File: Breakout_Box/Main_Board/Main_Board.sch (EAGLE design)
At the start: 31 parts, among them CN1 19PIN_LEMO, Q1 DMP3099L, Q2 DSS6060

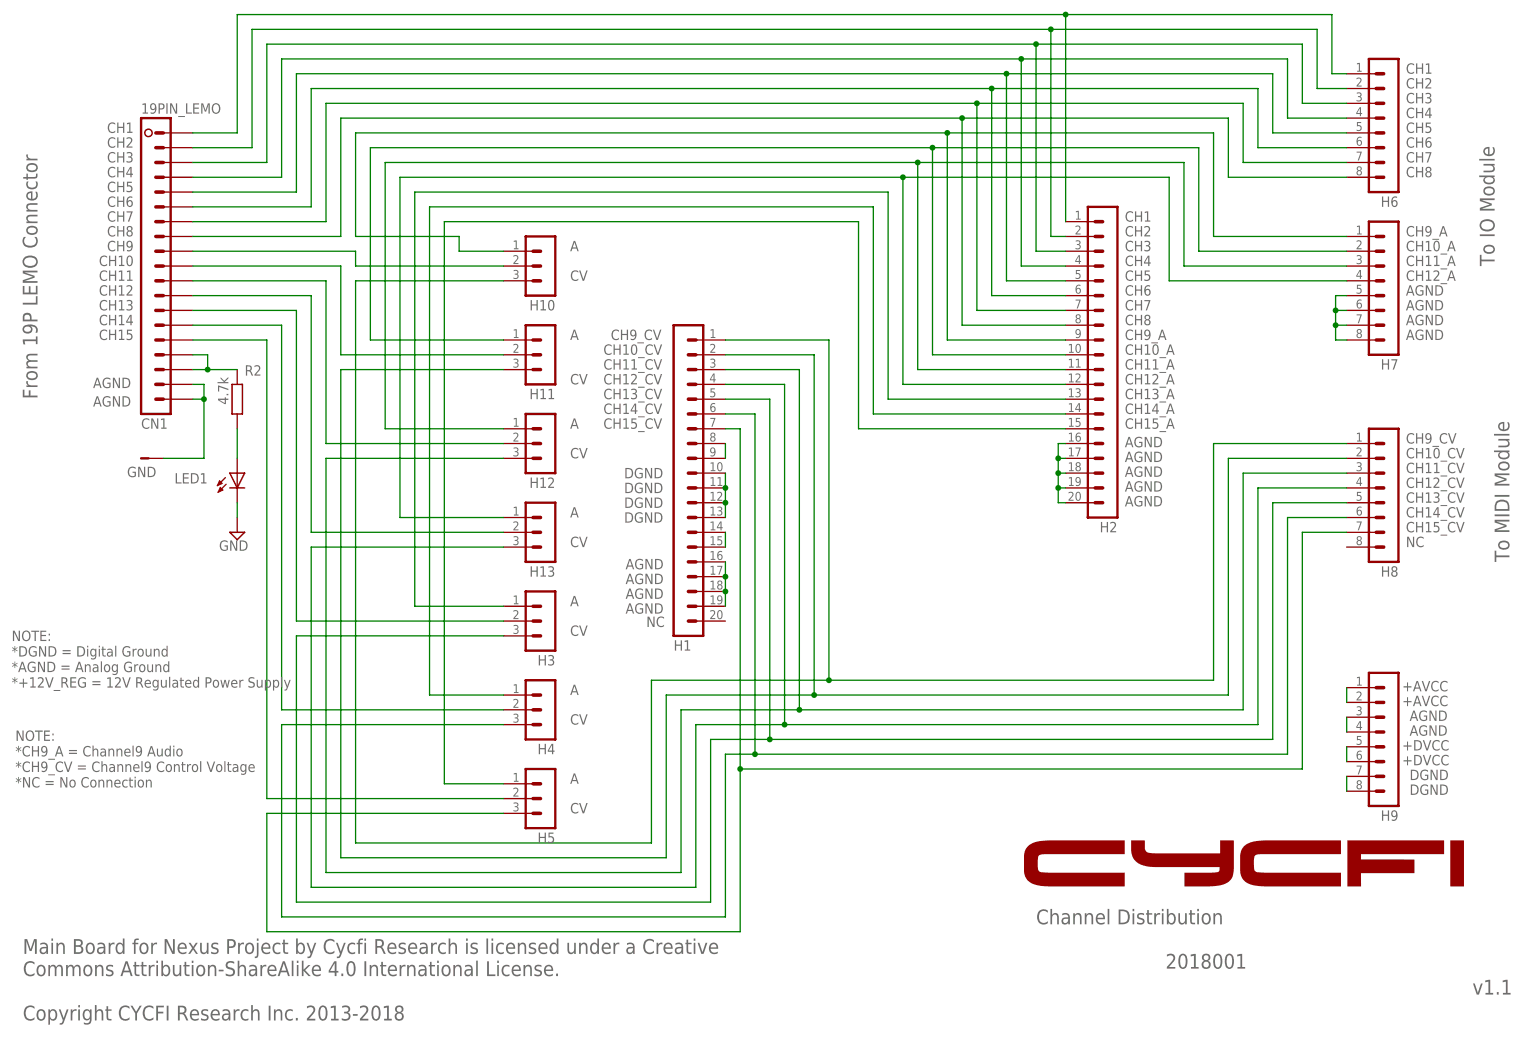
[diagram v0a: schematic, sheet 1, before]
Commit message: merge version_1.1 to devel
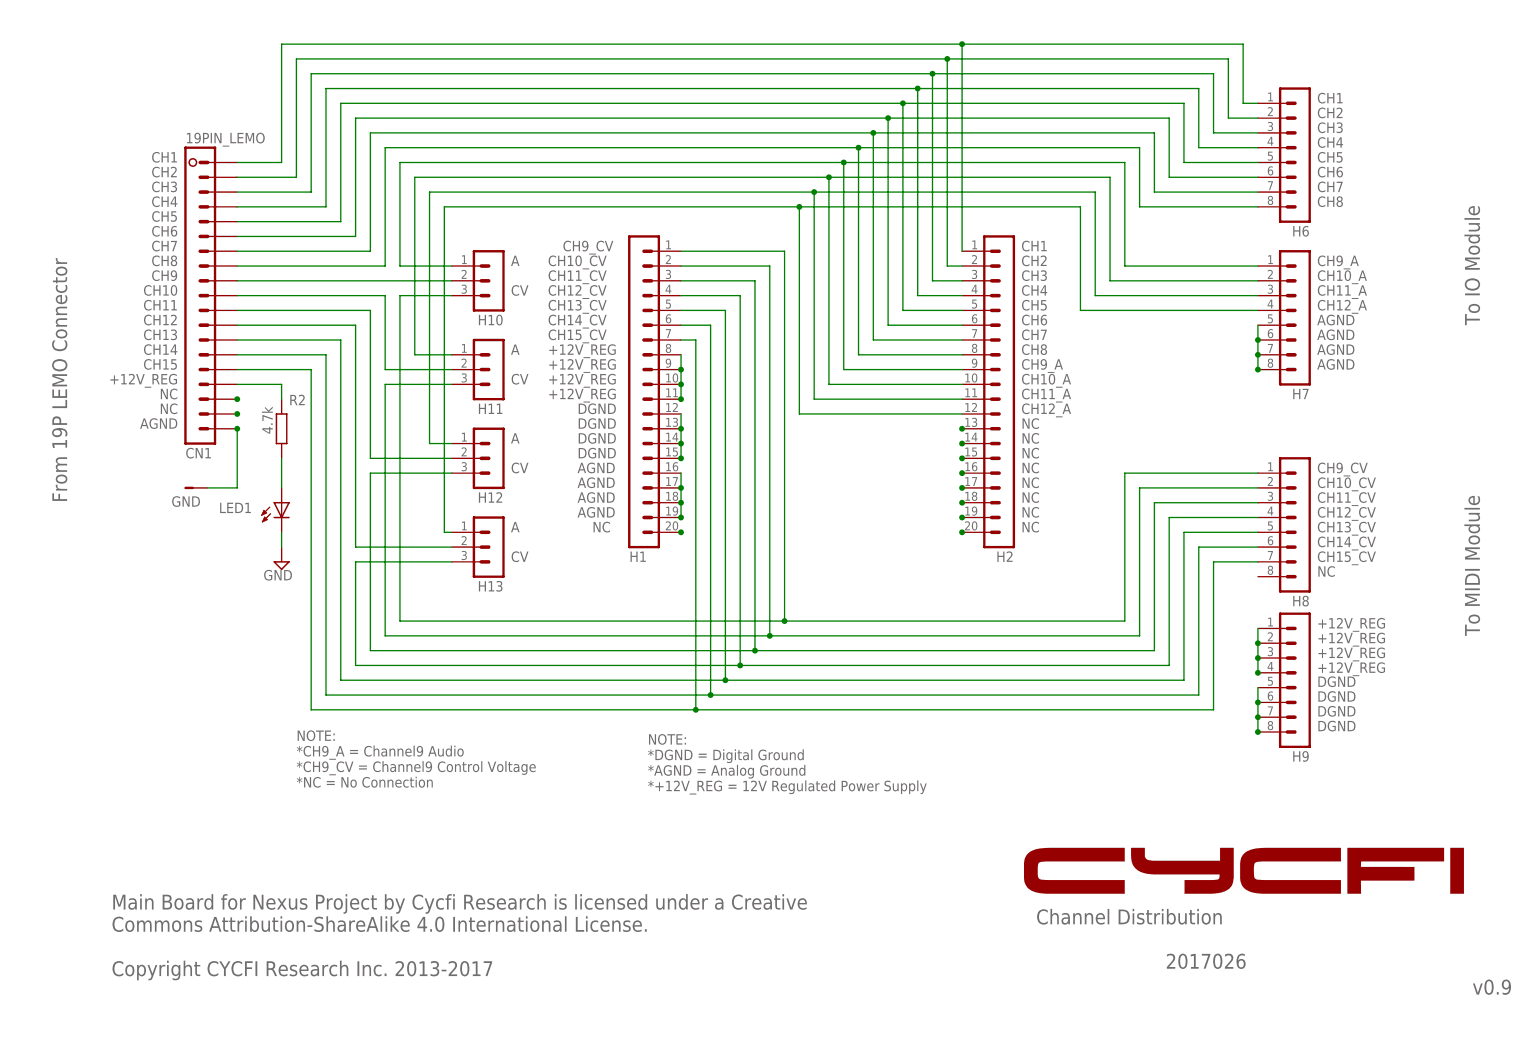
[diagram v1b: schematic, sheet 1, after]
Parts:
- removed C1, C3: 22uF, resistor:C-EUC0805
- removed C4: 1uF, resistor:C-EUC0603
- removed C5: 10uF, resistor:C-EUC0603
- removed C7: 1nF, resistor:C-EUC0402K
- removed H3, H4, H5: (no value), con-lstb:MA03-1_EDITED
- removed L2: 82uH, resistor:L-EU
- removed Q1: DMP3099L, CYCFI_semicon:P_MOSFET
- removed Q2: DSS6060, CYCFI_semicon:DSS60601MZ4-13
- removed R1: 1k, resistor:R-EU_R0402
- C2: value 470uF -> 0.1uF; device resistor:CPOL-EU140CLH-1010 -> resistor:C-EUC0603
- D1: value FM4004W -> FM4007W
- L1: value 1mH -> 100uH; device inductors:SDR -> resistor:L-EU
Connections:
- removed net +AVCC: C4.1, C5.1, C7.1, CN1.16, CN1.17, D1.A, H1.14, H1.15, H9.1, H9.2, Q2.E, R2.1
- removed net +DVCC: C3.1, H1.8, H1.9, H9.5, H9.6, L1.2
- removed net GND: C1.2, C2.-, C3.2, C4.2, C5.2, C6.-, C7.2, CN1.18, CN1.19, GND.P, H1.10, H1.11, H1.12, H1.13, H1.16, H1.17, H1.18, H1.19, H14.1, H2.16, H2.17, H2.18, H2.19, H2.20, H7.5, H7.6, H7.7, H7.8, H9.3, H9.4, H9.7, H9.8, LED1.C, Q1.G
- removed net N$33: H1.5, H3.3, H8.5
- removed net N$34: H1.6, H4.3, H8.6
- removed net N$35: H1.7, H5.3, H8.7
- removed net N$36: CN1.13, H3.2
- removed net N$37: CN1.14, H4.2
- removed net N$38: CN1.15, H5.2
- new net +12V_REG: C2.1, C6.+, CN1.16, H1.10, H1.11, H1.8, H1.9, H9.1, H9.2, H9.3, H9.4, L1.2, R2.1
- new net AGND: C2.2, C6.-, CN1.19, GND.P, H1.16, H1.17, H1.18, H1.19, H14.1, H7.5, H7.6, H7.7, H7.8, LED1.C
- new net DGND: H1.12, H1.13, H1.14, H1.15, H9.5, H9.6, H9.7, H9.8
- new net N$22: H2.19
- new net N$23: H2.20
- new net N$24: H1.20
- new net N$26: CN1.18
- new net N$31: D1.C, L1.1
- new net N$60: CN1.13, H1.5, H8.5
- new net N$61: CN1.14, H1.6, H8.6
- new net N$62: CN1.15, H1.7, H8.7
- new net N$9: CN1.17
- net N$1: no longer H3.1
- net N$17: no longer H5.1
- net N$19: now also H2.16; no longer C1.1, L1.1, L2.1, Q1.S
- net N$2: now also D1.A; no longer Q1.D
- net N$20: now also H2.17; no longer C2.+, Q2.B, R1.1
- net N$21: now also H2.18; no longer C6.+, D1.C, L2.2, Q2.C, R1.2
- net N$3: no longer H4.1
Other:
- note added: "2017026"
- note added: "Main Board for Nexus Project by Cycfi Research is licensed under a Creative Commons Attribution-ShareAlike 4.0 International License. Copyright CYCFI Research Inc. 2013-2017"
- note added: "NOTES: *+12V_REG = 12V Regulater Power Supply *AGND = Analog Ground *DGND= Digital Ground"
- note added: "v0.9"
- note added: "v0.92"
- note removed: "+AVCC"
- note removed: "+DVCC"
- note removed: "2018001"
- note removed: "CH13_A"
- note removed: "CH14_A"
- note removed: "CH15_A"
- note removed: "Main Board for Nexus Project by Cycfi Research is licensed under a Creative Commons Attribution-ShareAlike 4.0 International License. Copyright CYCFI Research Inc. 2013-2018"
- note removed: "NOTES: *+12V_REG = 12V Regulater Power Supply for Analog * +12_VREGD = 12V Regulater Power Supply for Digital *AGND = Analog Ground *DGND= Digital Ground"
- note removed: "v1.1"
- moved on the sheet: C6, CN1, D1, GND, H1, H10, H11, H12, H13, H2, H6, H7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

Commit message: reset devel
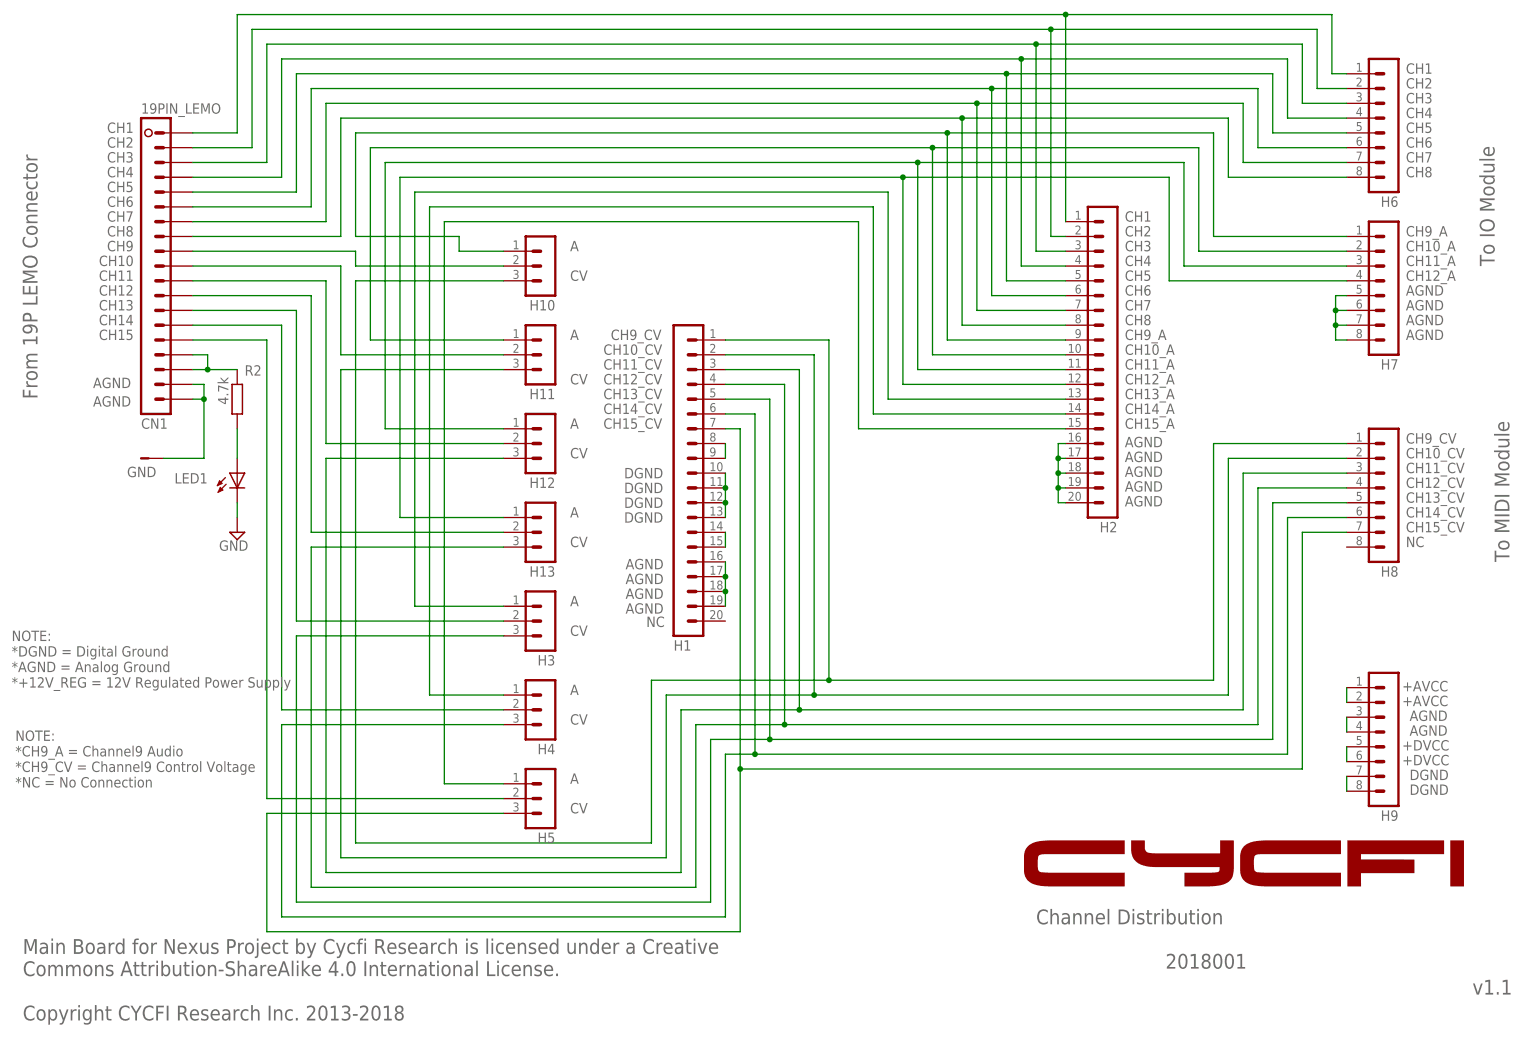
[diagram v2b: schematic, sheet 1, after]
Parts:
- added C1, C3: 22uF, resistor:C-EUC0805
- added C4: 1uF, resistor:C-EUC0603
- added C5: 10uF, resistor:C-EUC0603
- added C7: 1nF, resistor:C-EUC0402K
- added H3, H4, H5: (no value), con-lstb:MA03-1_EDITED
- added L2: 82uH, resistor:L-EU
- added Q1: DMP3099L, CYCFI_semicon:P_MOSFET
- added Q2: DSS6060, CYCFI_semicon:DSS60601MZ4-13
- added R1: 1k, resistor:R-EU_R0402
- C2: value 0.1uF -> 470uF; device resistor:C-EUC0603 -> resistor:CPOL-EU140CLH-1010
- D1: value FM4007W -> FM4004W
- L1: value 100uH -> 1mH; device resistor:L-EU -> inductors:SDR
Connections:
- removed net +12V_REG: C2.1, C6.+, CN1.16, H1.10, H1.11, H1.8, H1.9, H9.1, H9.2, H9.3, H9.4, L1.2, R2.1
- removed net AGND: C2.2, C6.-, CN1.19, GND.P, H1.16, H1.17, H1.18, H1.19, H14.1, H7.5, H7.6, H7.7, H7.8, LED1.C
- removed net DGND: H1.12, H1.13, H1.14, H1.15, H9.5, H9.6, H9.7, H9.8
- removed net N$22: H2.19
- removed net N$23: H2.20
- removed net N$24: H1.20
- removed net N$26 (its old number): CN1.18
- removed net N$31: D1.C, L1.1
- removed net N$60: CN1.13, H1.5, H8.5
- removed net N$61: CN1.14, H1.6, H8.6
- removed net N$62: CN1.15, H1.7, H8.7
- removed net N$9 (its old number): CN1.17
- new net +AVCC: C4.1, C5.1, C7.1, CN1.16, CN1.17, D1.A, H1.14, H1.15, H9.1, H9.2, Q2.E, R2.1
- new net +DVCC: C3.1, H1.8, H1.9, H9.5, H9.6, L1.2
- new net GND: C1.2, C2.-, C3.2, C4.2, C5.2, C6.-, C7.2, CN1.18, CN1.19, GND.P, H1.10, H1.11, H1.12, H1.13, H1.16, H1.17, H1.18, H1.19, H14.1, H2.16, H2.17, H2.18, H2.19, H2.20, H7.5, H7.6, H7.7, H7.8, H9.3, H9.4, H9.7, H9.8, LED1.C, Q1.G
- new net N$33: H1.5, H3.3, H8.5
- new net N$34: H1.6, H4.3, H8.6
- new net N$35: H1.7, H5.3, H8.7
- new net N$36: CN1.13, H3.2
- new net N$37: CN1.14, H4.2
- new net N$38: CN1.15, H5.2
- net N$1: now also H3.1
- net N$17: now also H5.1
- net N$19: now also C1.1, L1.1, L2.1, Q1.S; no longer H2.16
- net N$2: now also Q1.D; no longer D1.A
- net N$20: now also C2.+, Q2.B, R1.1; no longer H2.17
- net N$21: now also C6.+, D1.C, L2.2, Q2.C, R1.2; no longer H2.18
- net N$3: now also H4.1
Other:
- note added: "+AVCC"
- note added: "+DVCC"
- note added: "2018001"
- note added: "CH13_A"
- note added: "CH14_A"
- note added: "CH15_A"
- note added: "Main Board for Nexus Project by Cycfi Research is licensed under a Creative Commons Attribution-ShareAlike 4.0 International License. Copyright CYCFI Research Inc. 2013-2018"
- note added: "NOTES: *+12V_REG = 12V Regulater Power Supply for Analog * +12_VREGD = 12V Regulater Power Supply for Digital *AGND = Analog Ground *DGND= Digital Ground"
- note added: "v1.1"
- note removed: "2017026"
- note removed: "Main Board for Nexus Project by Cycfi Research is licensed under a Creative Commons Attribution-ShareAlike 4.0 International License. Copyright CYCFI Research Inc. 2013-2017"
- note removed: "NOTES: *+12V_REG = 12V Regulater Power Supply *AGND = Analog Ground *DGND= Digital Ground"
- note removed: "v0.9"
- note removed: "v0.92"
- moved on the sheet: C6, CN1, D1, GND, H1, H10, H11, H12, H13, H2, H6, H7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
